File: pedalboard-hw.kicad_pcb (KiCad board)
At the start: 4 copper layers, 174 x 111 mm, 120 parts, among them IC1 TAC5212IRGER, J10 USB-A HOST, J11 CM5 BOOT, J13 Headphones 3.5mm, J16 CM5 UART DEBUG, J18 GUITAR INPUT, J19 LINE OUT LEFT, J20 LINE OUT RIGHT, J21 UI LINK 2x5, J22 BALANCED LINE INPUT, J6 Screw_Terminal_01x02, J7 Barrel_Jack_MountingPin, J9 USB-C SERVICE, Q1 FDS4435BZ, SW11 EM-02-Q, U10 AP22653, U11 TPD2E2U06DCK, U13 LT3042, U14 OPA1656ID, U15 TPS7A20, U16 TPD2E2U06DCK, U6 TLVM13660

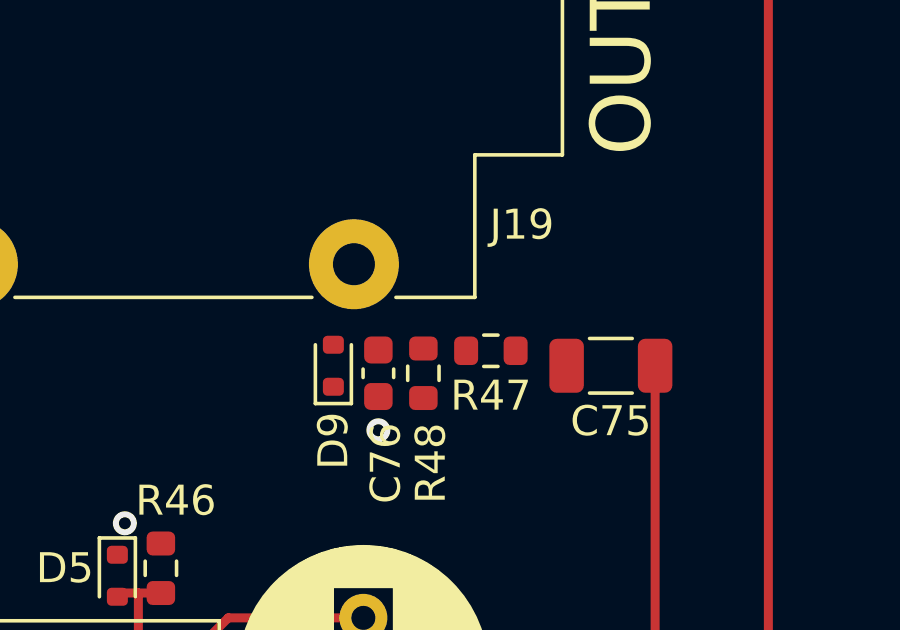
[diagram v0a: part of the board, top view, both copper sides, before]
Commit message: bit more routing.
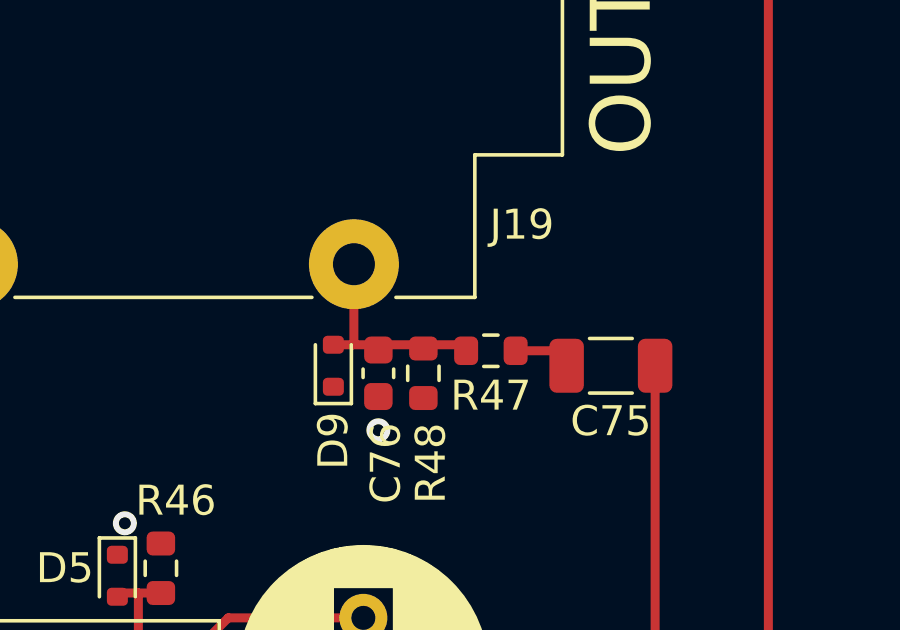
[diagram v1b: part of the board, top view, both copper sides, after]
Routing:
- net Net-(D9-A2): track 0.00 -> 7.21 mm
- net Net-(C75-Pad2): track 0.00 -> 1.91 mm
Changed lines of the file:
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@@
+	)
+	(segment
+		(start 34.685 92.765)
+		(end 34.65 92.8)
+		(width 0.3)
+		(layer "F.Cu")
+		(net "Net-(D9-A2)")
+	)
+	(segment
+		(start 38.225 92.8)
+		(end 38.425 93)
+		(width 0.3)
+		(layer "F.Cu")
+		(net "Net-(D9-A2)")
+	)
+	(segment
+		(start 34 92.8)
+		(end 34.65 92.8)
+		(width 0.3)
+		(layer "F.Cu")
+		(net "Net-(D9-A2)")
+	)
+	(segment
+		(start 34.685 90.115)
+		(end 34.685 92.765)
+		(width 0.3)
+		(layer "F.Cu")
+		(net "Net-(D9-A2)")
+	)
+	(segment
+		(start 34.65 92.8)
+		(end 38.225 92.8)
+		(width 0.3)
+		(layer "F.Cu")
+		(net "Net-(D9-A2)")
 	)
 	(segment
@@
 	)
 	(segment
+		(start 40.075 93)
+		(end 41.275 93)
+		(width 0.3)
+		(layer "F.Cu")
+		(net "Net-(C75-Pad2)")
+	)
+	(segment
+		(start 41.275 93)
+		(end 41.775 93.5)
+		(width 0.3)
+		(layer "F.Cu")
+		(net "Net-(C75-Pad2)")
+	)
+	(segment
